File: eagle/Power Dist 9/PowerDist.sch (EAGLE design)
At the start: 14 parts

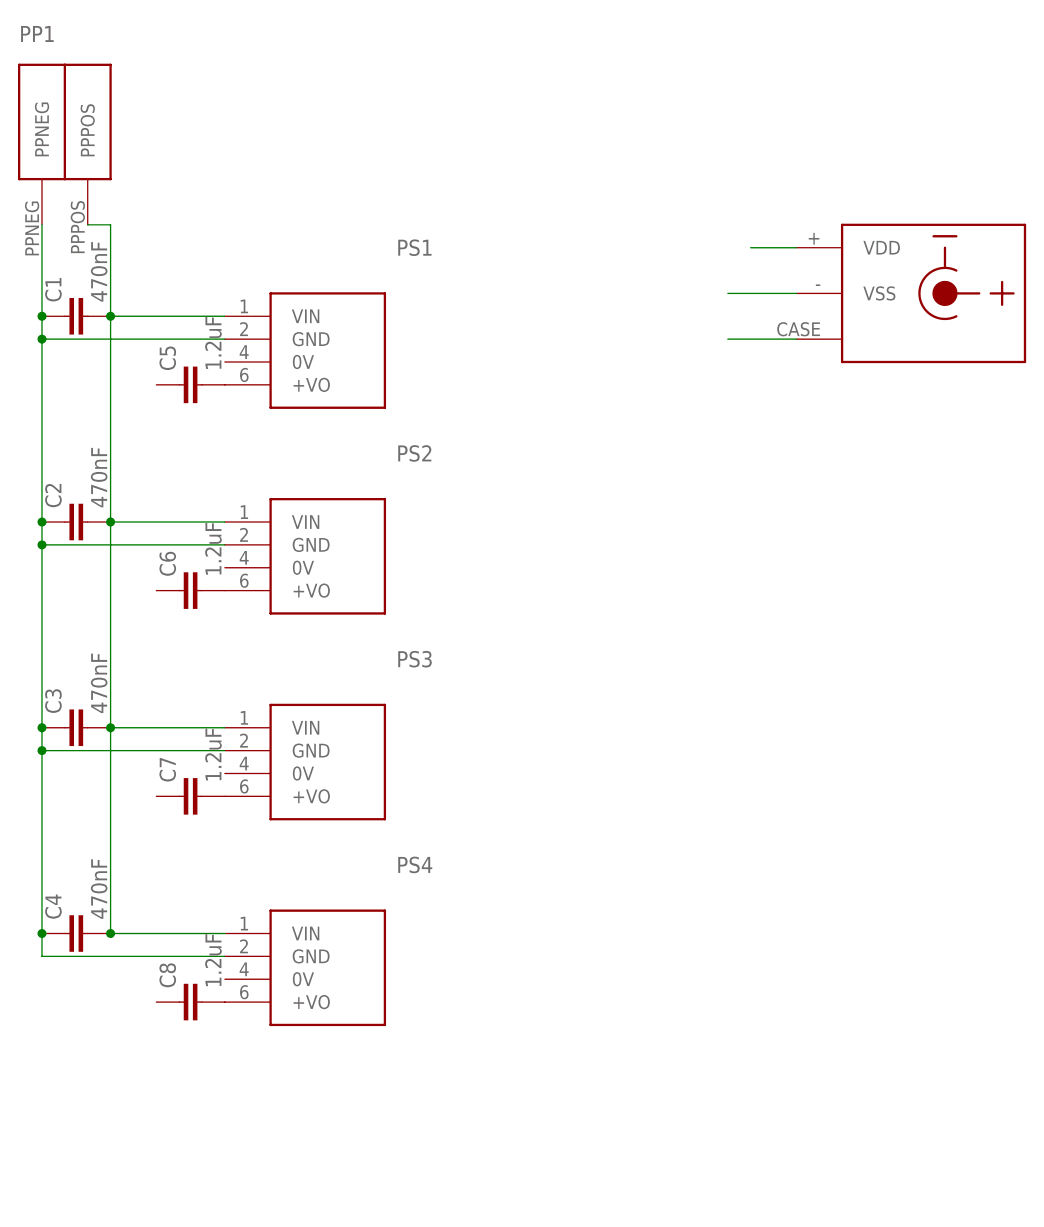
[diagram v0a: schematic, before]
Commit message: latest
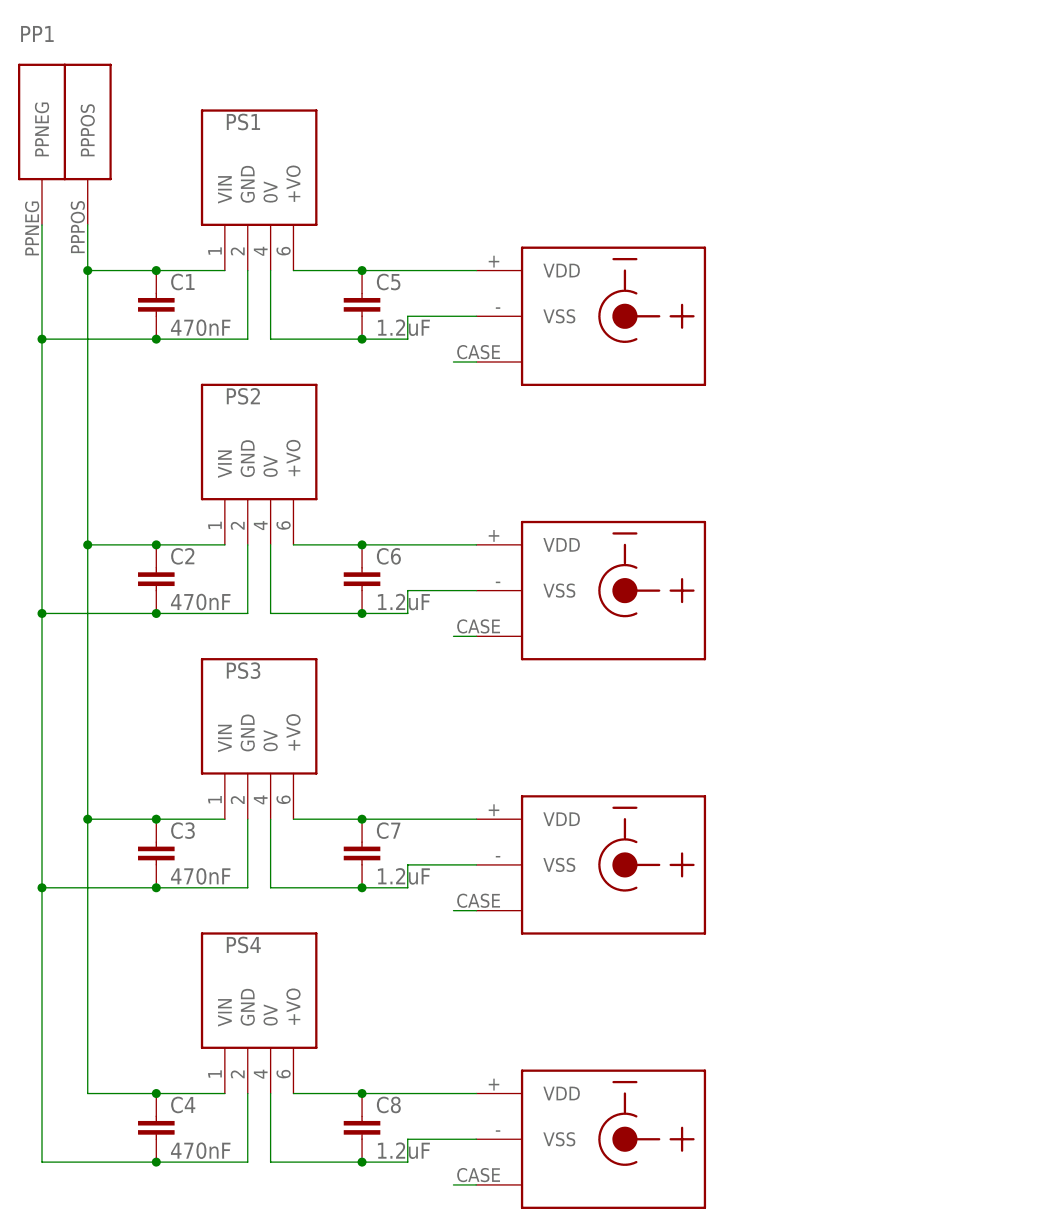
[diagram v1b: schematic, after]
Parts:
- added U$2, U$3, U$4: CUI_PJ-102A, con-dc-jack:CUI_PJ-102A
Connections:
- removed net GND2: U$1.VSS
- removed net VCC2: U$1.VDD
- new net CASE1: U$2.@3
- new net CASE2: U$3.@3
- new net CASE3: U$4.@3
- new net N$10: C8.2, PS4.0V, U$4.VSS
- new net N$7: C5.2, PS1.0V, U$1.VSS
- new net N$8: C6.2, PS2.0V, U$2.VSS
- new net N$9: C7.2, PS3.0V, U$3.VSS
- net N$1: now also PP1.PPPOS, PS1.VIN, PS2.VIN, PS3.VIN, PS4.VIN; no longer PP1.PPNEG, PS1.GND, PS2.GND, PS3.GND, PS4.GND
- net N$2: now also PP1.PPNEG, PS1.GND, PS2.GND, PS3.GND, PS4.GND; no longer PP1.PPPOS, PS1.VIN, PS2.VIN, PS3.VIN, PS4.VIN
- net N$3: now also C5.1, U$1.VDD; no longer C5.2
- net N$4: now also C6.1, U$2.VDD; no longer C6.2
- net N$5: now also C7.1, U$3.VDD; no longer C7.2
- net N$6: now also C8.1, U$4.VDD; no longer C8.2
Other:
- moved on the sheet: C1, C2, C3, C4, C5, C6, C7, C8, PS1, PS2, PS3, PS4
